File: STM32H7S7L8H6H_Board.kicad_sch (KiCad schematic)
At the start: 142 parts, among them IC1 STM32H7S7L8H6H, IC2 SDRAM_IS42S16320F-6TL, J1 LPUART1_Headers, J10 Power Select Jumpers, J11 Debug_Pins, J12 User Button Jumper, J13 USB_B_Micro, J14 USB_B_Micro, J15 Debug_Pins, J2 I2C1_Headers, J3 Power Pins, J4 Pin_Headers, J5 SPI1_Headers, J6 Power Select Jumpers, J7 Coin Battery Jumper, J8 BOOT0_Jumper, J9 BOOT0_Jumper, U1 STM32WL55CCU6, U3 LD1117S18TR_SOT223, U4 FT230XS, U5 USBLC6-2SC6, Y1 ABM3B-32.000MHZ-8-R30-B1U-T, Y2 Clock_ECS-327MVATX-7-CN-TR, Y4 Oscillator_ASE-50.000MHZ-L-R-T

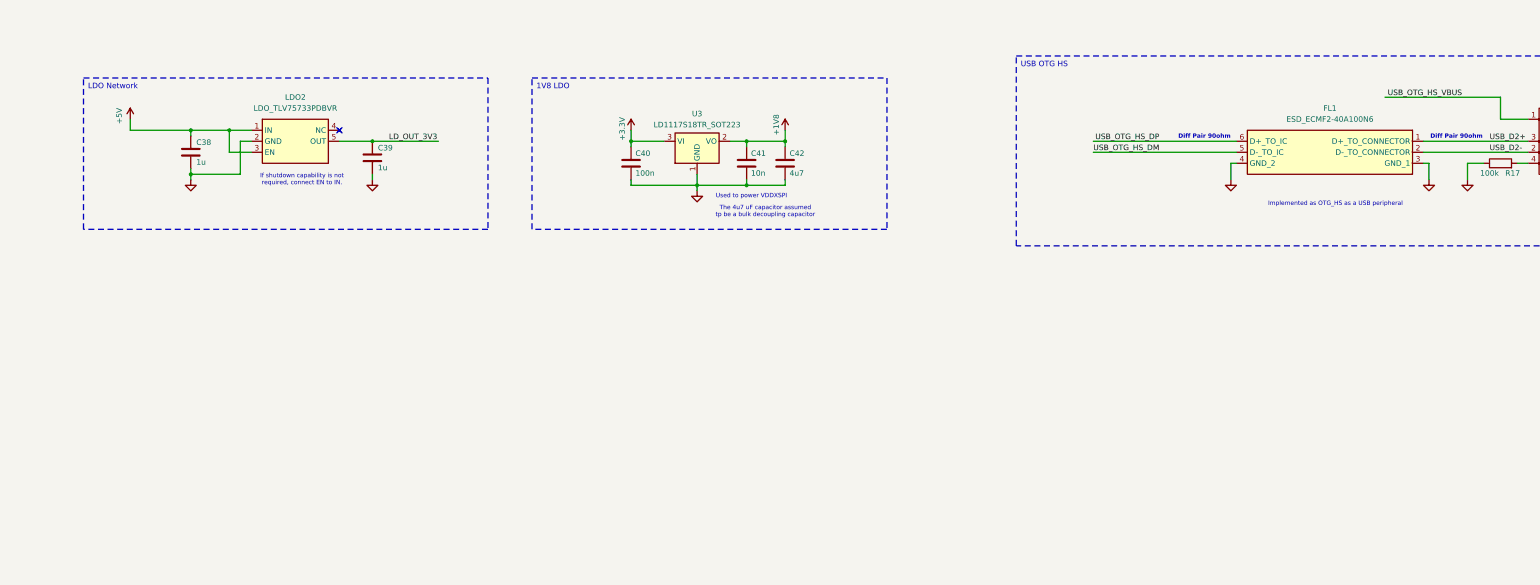
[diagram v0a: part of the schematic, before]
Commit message: Update
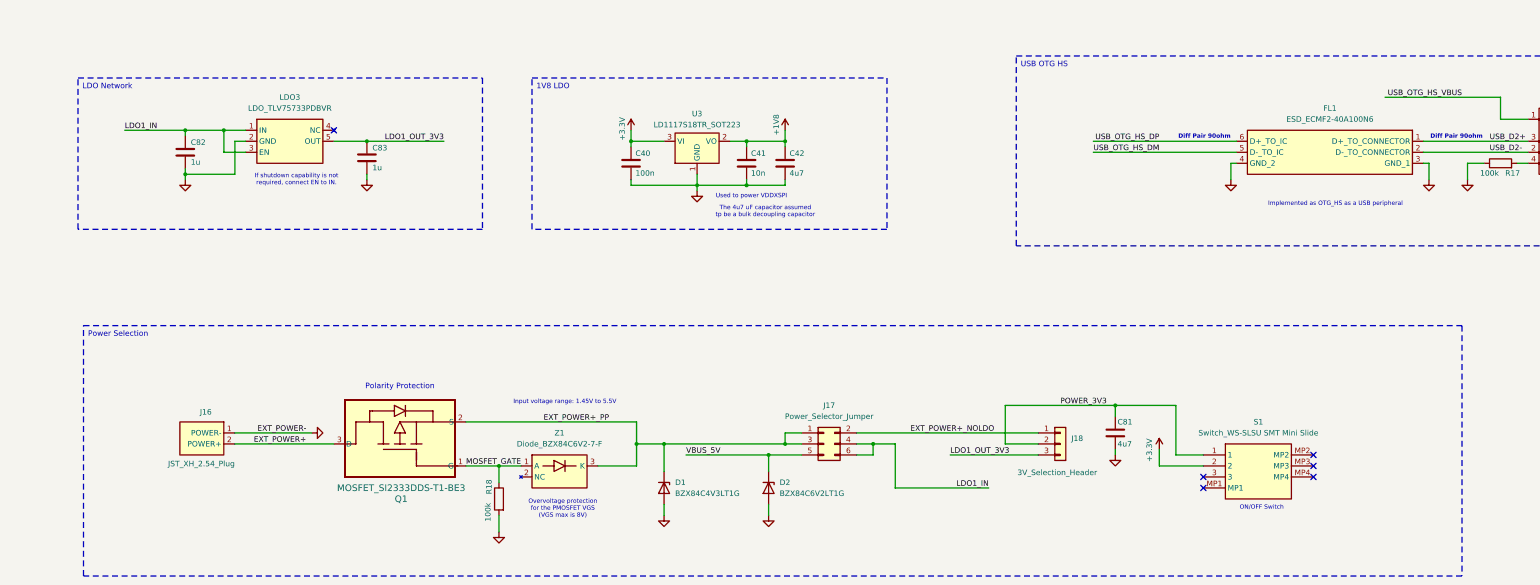
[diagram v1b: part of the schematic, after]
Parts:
- removed C38, C39: 1u, Capacitor_SMD:C_0805_2012Metric_Pad1.18x1.45mm_HandSolder, symbol Device:C
- removed LDO2: LDO_TLV75733PDBVR, Personal_Project:LDO_SOT95P280X145-5N, symbol Personal_Projects:LDO_TLV75733PDBVR
- added C81: 4u7, Capacitor_SMD:C_0603_1608Metric_Pad1.08x0.95mm_HandSolder, symbol Device:C
- added C82, C83: 1u, Capacitor_SMD:C_0805_2012Metric_Pad1.18x1.45mm_HandSolder, symbol Device:C
- added D1: BZX84C4V3LT1G, Package_TO_SOT_SMD:SOT-23, symbol Diode:BZX84Cxx
- added D2: BZX84C6V2LT1G, Package_TO_SOT_SMD:SOT-23, symbol Diode:BZX84Cxx
- added J16: JST_XH_2.54_Plug, Personal_Project:Connector_Power2pin_SHDRRA2W80P0X250_1X2_740X1150X610P, symbol Personal_Projects:Connector_Power2pin_JST_XH_2.54_Plug
- added J17: Power_Selector_Jumper, Connector_PinHeader_2.54mm:PinHeader_2x03_P2.54mm_Vertical, symbol Connector_Generic:Conn_02x03_Odd_Even
- added J18: 3V_Selection_Header, Connector_PinHeader_2.54mm:PinHeader_1x03_P2.54mm_Vertical, symbol Connector_Generic:Conn_01x03
- added LDO3: LDO_TLV75733PDBVR, Personal_Project:LDO_SOT95P280X145-5N, symbol Personal_Projects:LDO_TLV75733PDBVR
- added Q1: MOSFET_SI2333DDS-T1-BE3, Personal_Project:MOSFET_ SI2333DDS_SOT_DS-T1-BE3_VIS, symbol Personal_Projects:MOSFET_SI2333DDS-T1-BE3
- added R18: 100k, Resistor_SMD:R_0603_1608Metric_Pad0.98x0.95mm_HandSolder, symbol Device:R
- added S1: Switch_WS-SLSU SMT Mini Slide, Personal_Project:Switch_WS-SLSU SMT Mini Slide, symbol Personal_Projects:Switch_WS-SLSU SMT Mini Slide
- added Z1: Diode_BZX84C6V2-7-F, Personal_Project:Diode_BZX84C6V2_SOT96P240X110-3N, symbol Personal_Projects:Diode_BZX84C6V2-7-F
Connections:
- net +3.3V: now also S1.2
- net GND: now also C81.2, C82.2, C83.2, D1.1 (A), D2.1 (A), J16.1 (POWER-), LDO3.2 (GND), R18.2
- net VBUS_5V: now also D2.3 (K), J17.5 (Pin_5)
- new net EXT_POWER+: J16.2 (POWER+), Q1.3 (D)
- new net EXT_POWER+_NOLDO: J17.2 (Pin_2), J18.1 (Pin_1)
- new net EXT_POWER+_PP: D1.3 (K), J17.1 (Pin_1), J17.3 (Pin_3), Q1.2 (S), Z1.3 (K)
- new net LDO1_IN: C82.1, J17.4 (Pin_4), J17.6 (Pin_6), LDO3.1 (IN), LDO3.3 (EN)
- new net LDO1_OUT_3V3: C83.1, J18.3 (Pin_3), LDO3.5 (OUT)
- new net MOSFET_GATE: Q1.1 (G), R18.1, Z1.1 (A)
- new net POWER_3V3: C81.1, J18.2 (Pin_2), S1.1
- no-connect marks 15 -> 20
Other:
- note added: "Input voltage range: 1.45V to 5.5V"
- note added: "ON/OFF Switch"
- note added: "Overvoltage protection for the PMOSFET VGS (VGS max is 8V)"
- note added: "Polarity Protection"
